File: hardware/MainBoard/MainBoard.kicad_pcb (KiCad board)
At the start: 4 copper layers, 28 x 58.4 mm, 56 parts, among them J1 Conn_02x16_Top_Bottom, J2 Conn_02x16_Top_Bottom, J3 USB_C_Receptacle_USB2.0_16P, J4 En_A, J5 En_B, J6 Micro_SD_Card_Det2, J7 Conn_02x16_Top_Bottom, Q1 MMBT2222A, Q2 FDN340P, Q3 FDN340P, U1 ESP32-S3-WROOM-1, U2 AMS1117-3.3, U3 AMS1117-5.0

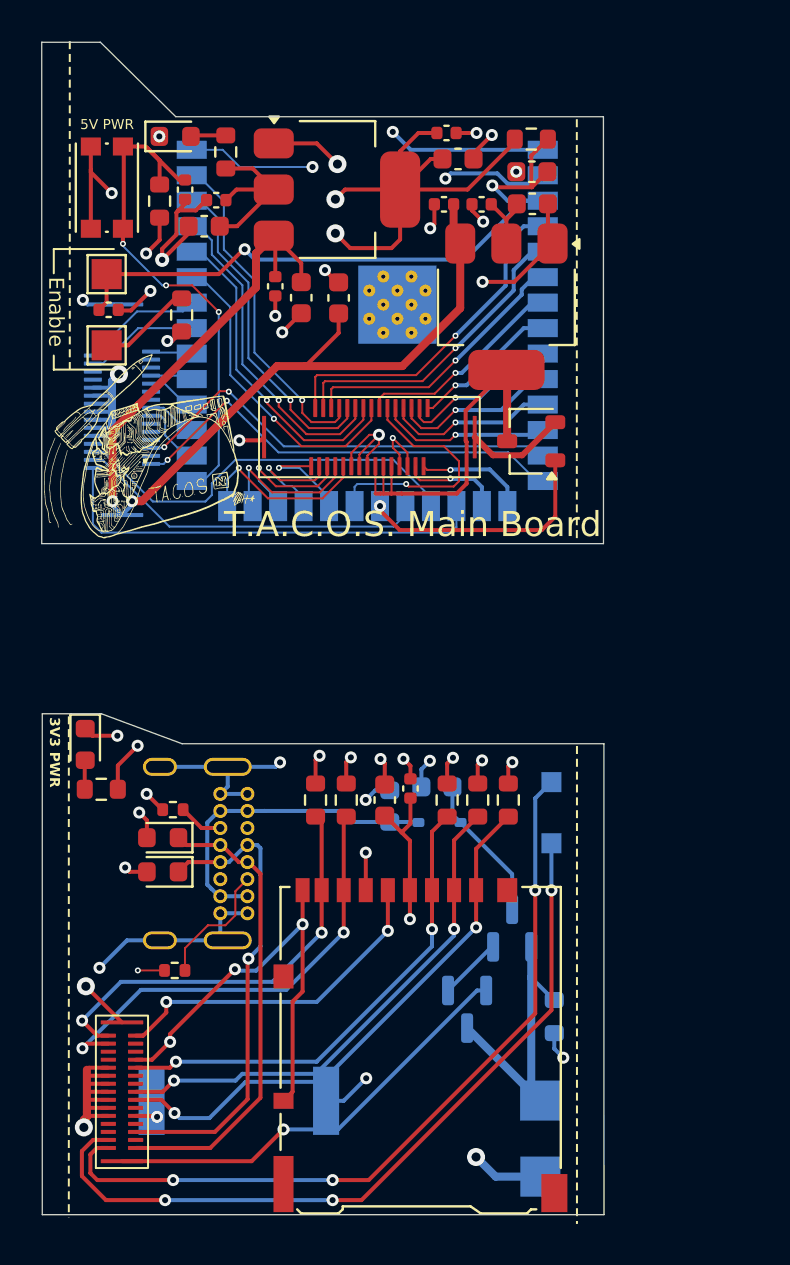
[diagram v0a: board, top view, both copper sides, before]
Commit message: fixed main hat
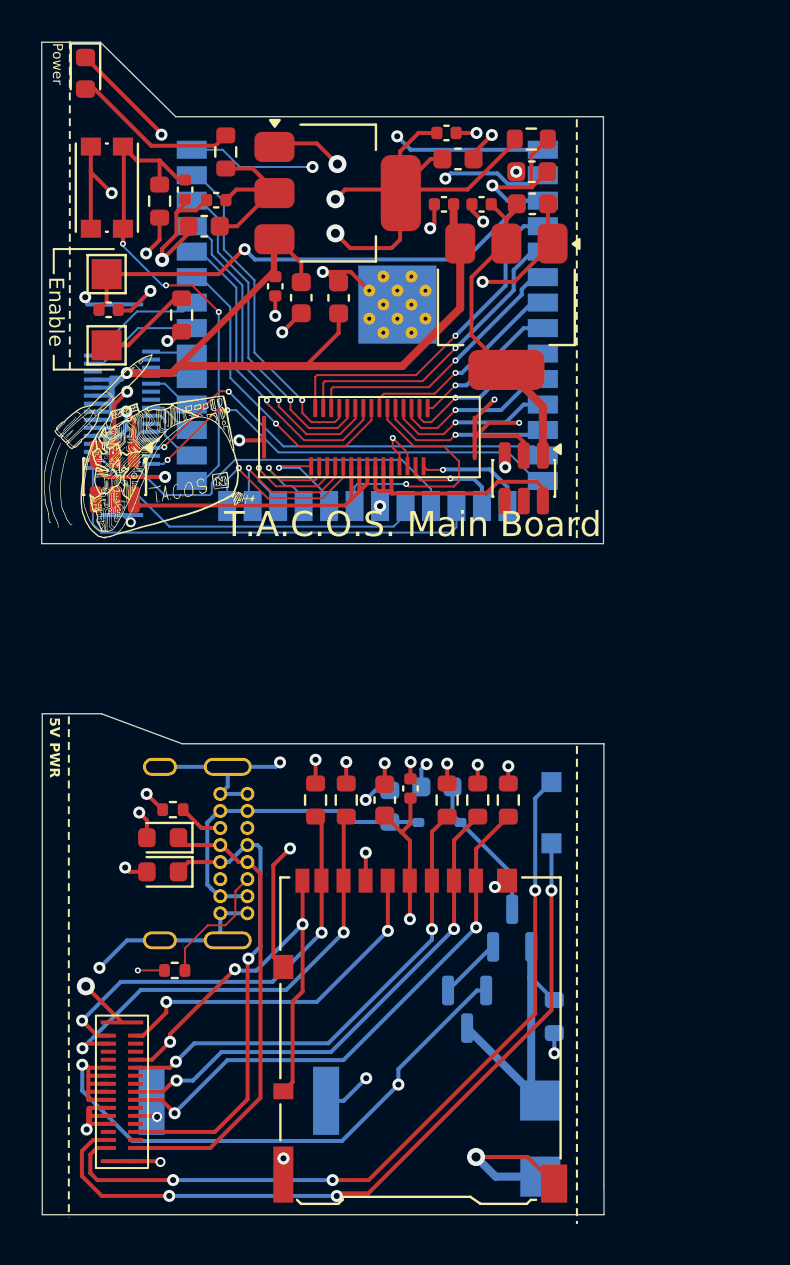
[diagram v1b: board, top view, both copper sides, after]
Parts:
- removed D2: PWRLED, LED_SMD:LED_0603_1608Metric
- removed Q1: MMBT2222A, Package_TO_SOT_SMD:SOT-23W
- removed R3: 75, Resistor_SMD:R_0603_1608Metric
- added U4: TPS22917DBV, Package_TO_SOT_SMD:SOT-23-6, F.Cu at (66.1, 72.9)
- added U5: TPS22917DBV, Package_TO_SOT_SMD:SOT-23-6, F.Cu at (86.5, 73.0)
- U1: footprint RF_Module:ESP32-S3-WROOM-1 -> RF_Module:ESP32-S3-WROOM-1U
- moved D1 5.47 mm to (64.7, 52.8), turned to -90 degrees
- moved U1 3.15 mm to (78.7, 65.0)
- moved J6 0.47 mm to (81.4, 100.8)
- moved U2 0.18 mm to (77.2, 58.8)
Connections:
- C13 pad 1: CONN_19 -> CONN_18
- C15 pad 1: CONN_19 -> CONN_18
- C2 pad 1: CONN_19 -> CONN_18
- C3 pad 1: CONN_19 -> CONN_18
- C4 pad 1: VIN -> CONN_21
- C5 pad 1: VIN -> CONN_21
- C6 pad 1: CONN_19 -> CONN_18
- C7 pad 1: CONN_19 -> CONN_18
- C8 pad 1: VIN -> CONN_21
- C9 pad 1: VIN -> CONN_21
- J1 pad 20: CONN_19 -> CONN_18
- J1 pad 21: CONN_19 -> CONN_18
- J1 pad 22: CONN_19 -> CONN_21
- J1 pad 23: CONN_19 -> CONN_21
- J1 pad 24: CONN_19 -> CONN_21
- J1 pad 25: CONN_19 -> CONN_21
- J1 pad 26: CONN_19 -> CONN_21
- J1 pad 27: CONN_26 -> CONN_21
- J2 pad 10: CONN_19 -> CONN_21
- J2 pad 11: CONN_19 -> CONN_21
- J2 pad 12: CONN_26 -> CONN_21
- J2 pad 5: CONN_19 -> CONN_18
- J2 pad 6: CONN_19 -> CONN_18
- J2 pad 7: CONN_19 -> CONN_21
- J2 pad 8: CONN_19 -> CONN_21
- J2 pad 9: CONN_19 -> CONN_21
- J6 pad 4: CONN_19 -> CONN_18
- J7 pad 20: VCC_5V -> CONN_5V
- J7 pad 21: VCC_5V -> CONN_5V
- J7 pad 22: VCC_5V -> CONN_5V
- J7 pad 23: CONN_19 -> CONN_3V3
- J7 pad 24: CONN_19 -> CONN_3V3
- J7 pad 25: CONN_19 -> CONN_3V3
- Q3 pad 2: VIN -> CONN_21
- R1 pad 1: CONN_19 -> CONN_18
- R10 pad 1: CONN_19 -> CONN_18
- R11 pad 1: CONN_19 -> CONN_18
- R12 pad 1: CONN_19 -> CONN_18
- R2 pad 1: CONN_19 -> CONN_18
- R6 pad 1: CONN_19 -> CONN_18
- R7 pad 1: CONN_19 -> CONN_18
- R8 pad 1: CONN_19 -> CONN_18
- R9 pad 1: CONN_19 -> CONN_18
- U1 pad 2: CONN_19 -> CONN_18
- U2 pad 2: CONN_19 -> CONN_18
- U2 pad 3: VIN -> CONN_21
- U3 pad 3: VIN -> CONN_21
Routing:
- net CONN_21: track 0.00 -> 82.9 mm, vias 0 -> 3
- net CONN_19: track 82.2 -> 0.00 mm, vias 14 -> 0
- net VIN: track 74.6 -> 0.00 mm, vias 3 -> 0
- net CONN_18: track 0.00 -> 66.9 mm, vias 0 -> 13
- net LIPO GND: track 97.0 -> 128.2 mm, vias 35 -> 42
- net CONN_3V3: track 0.00 -> 16.0 mm
- net HATS_ENABLE: track 12.4 -> 23.5 mm, vias 1 -> 3
- net VCC_5V: track 24.8 -> 16.1 mm, vias 1 -> 0
- net CONN_5V: track 5.08 -> 13.2 mm
- net Net-(D1-A): track 1.76 -> 8.38 mm
- net Net-(D2-A): track 1.46 -> 0.00 mm
- net GPIO0: track 26.3 -> 25.4 mm
- added copper zone on In2.Cu, net CONN_18
- removed copper zone on In2.Cu, net CONN_19
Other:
- board text removed: "3V3 PWR"
